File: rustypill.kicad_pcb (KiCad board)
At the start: 2 copper layers, 69 x 48 mm, 50 parts, among them IC1 DS3231, J1 USB, J2 PROG, J3 GPIOB, J4 GPIOA, J5 LCD1602, J6 IDC_10P, J7 I2C, M2 MountingHole_2.7mm_M2.5, M3 MountingHole_2.7mm_M2.5, M4 MountingHole_2.7mm_M2.5, SW1 Reset, U1 AMS1117-3.3, U2 AT24C512C-SSHD-T, U3 ESP-12F, U4 STM32F103C8Tx, Y1 8MHz

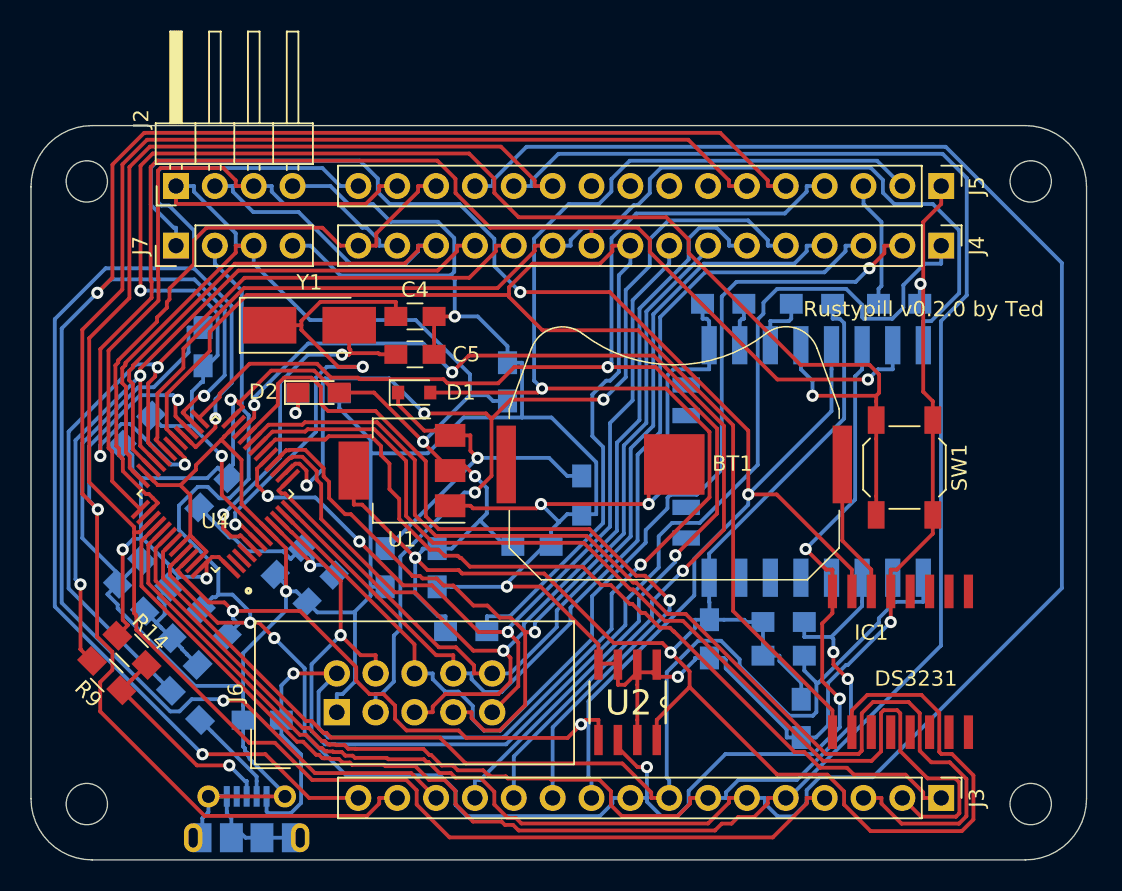
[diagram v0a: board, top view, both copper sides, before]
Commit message: v0.2.0
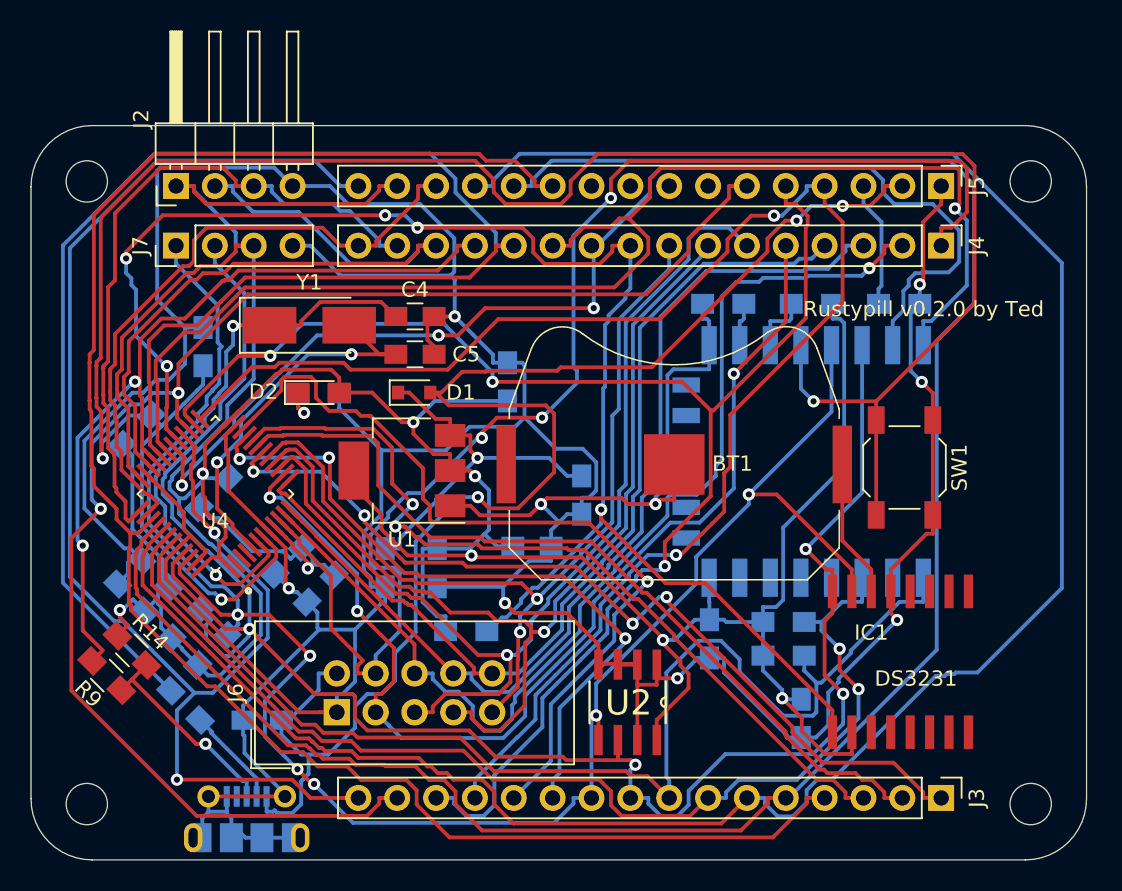
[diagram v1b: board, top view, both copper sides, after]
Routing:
- net A11: track 60.8 -> 102.1 mm, vias 1 -> 0
- net IC_RST: track 107.0 -> 143.9 mm
- net B13: track 125.6 -> 96.2 mm
- net GND: track 313.5 -> 334.8 mm, vias 8 -> 9
- net B14: track 118.0 -> 97.3 mm
- net B2: track 74.9 -> 54.4 mm, vias 0 -> 2
- net B9: track 143.3 -> 123.0 mm, vias 4 -> 6
- net VPP: track 114.6 -> 95.0 mm
- net +3V3: track 265.9 -> 249.8 mm
- net B1: track 70.0 -> 54.2 mm
- net B11: track 67.8 -> 54.0 mm, vias 3 -> 1
- net A10: track 75.3 -> 87.2 mm, vias 0 -> 1
- net A9: track 88.4 -> 78.8 mm
- net B10: track 54.8 -> 46.1 mm, vias 1 -> 3
- net 32KHZ_IN: track 110.7 -> 102.2 mm, vias 0 -> 5
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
